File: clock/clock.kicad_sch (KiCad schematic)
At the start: 4 parts

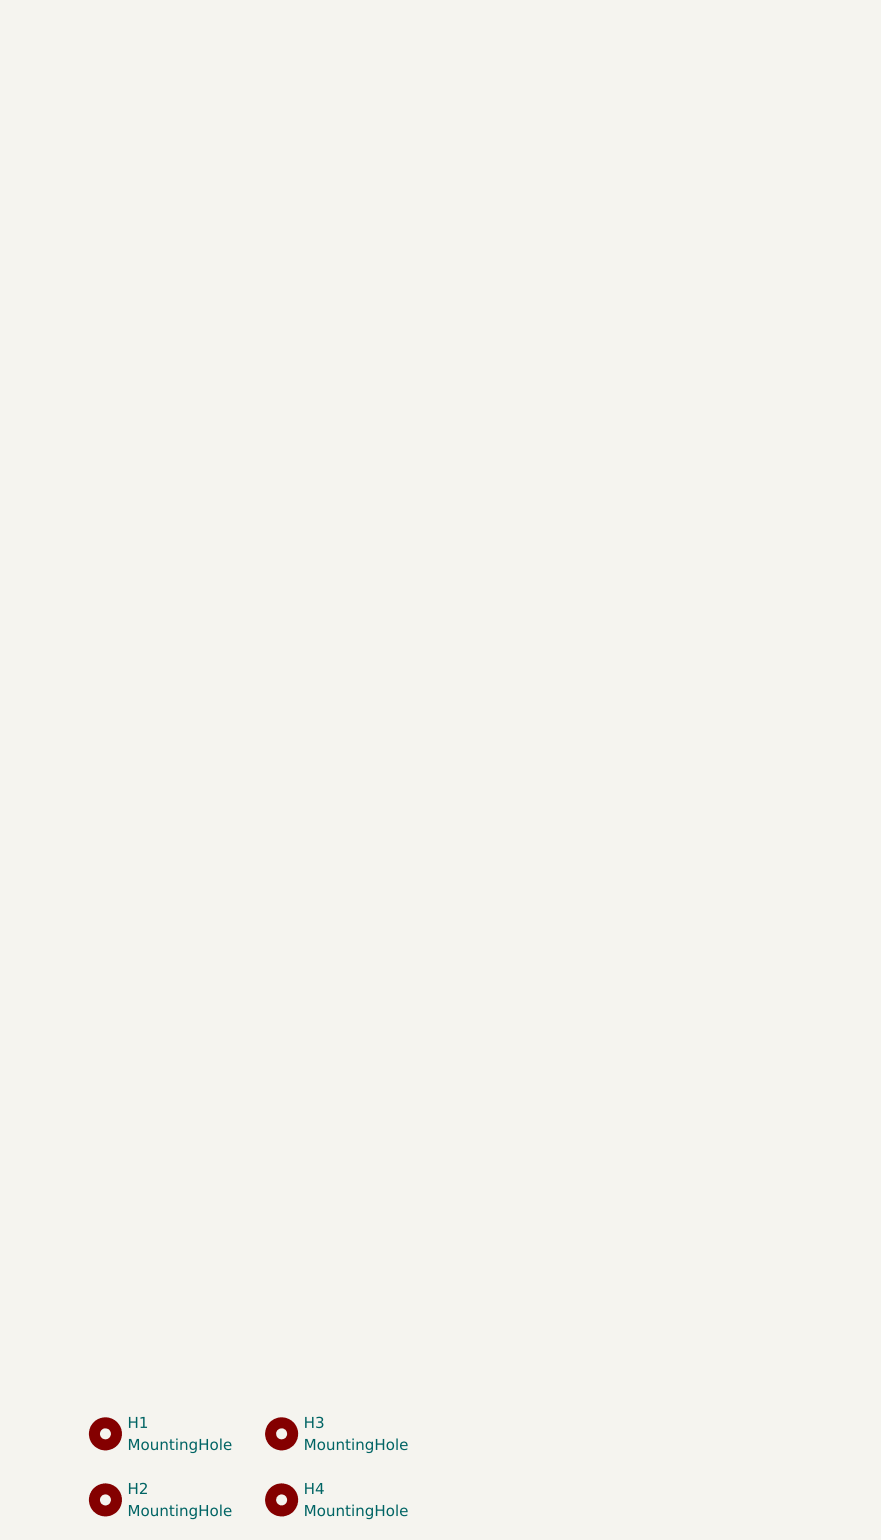
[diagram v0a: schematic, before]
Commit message: kinda week 2 deliverables
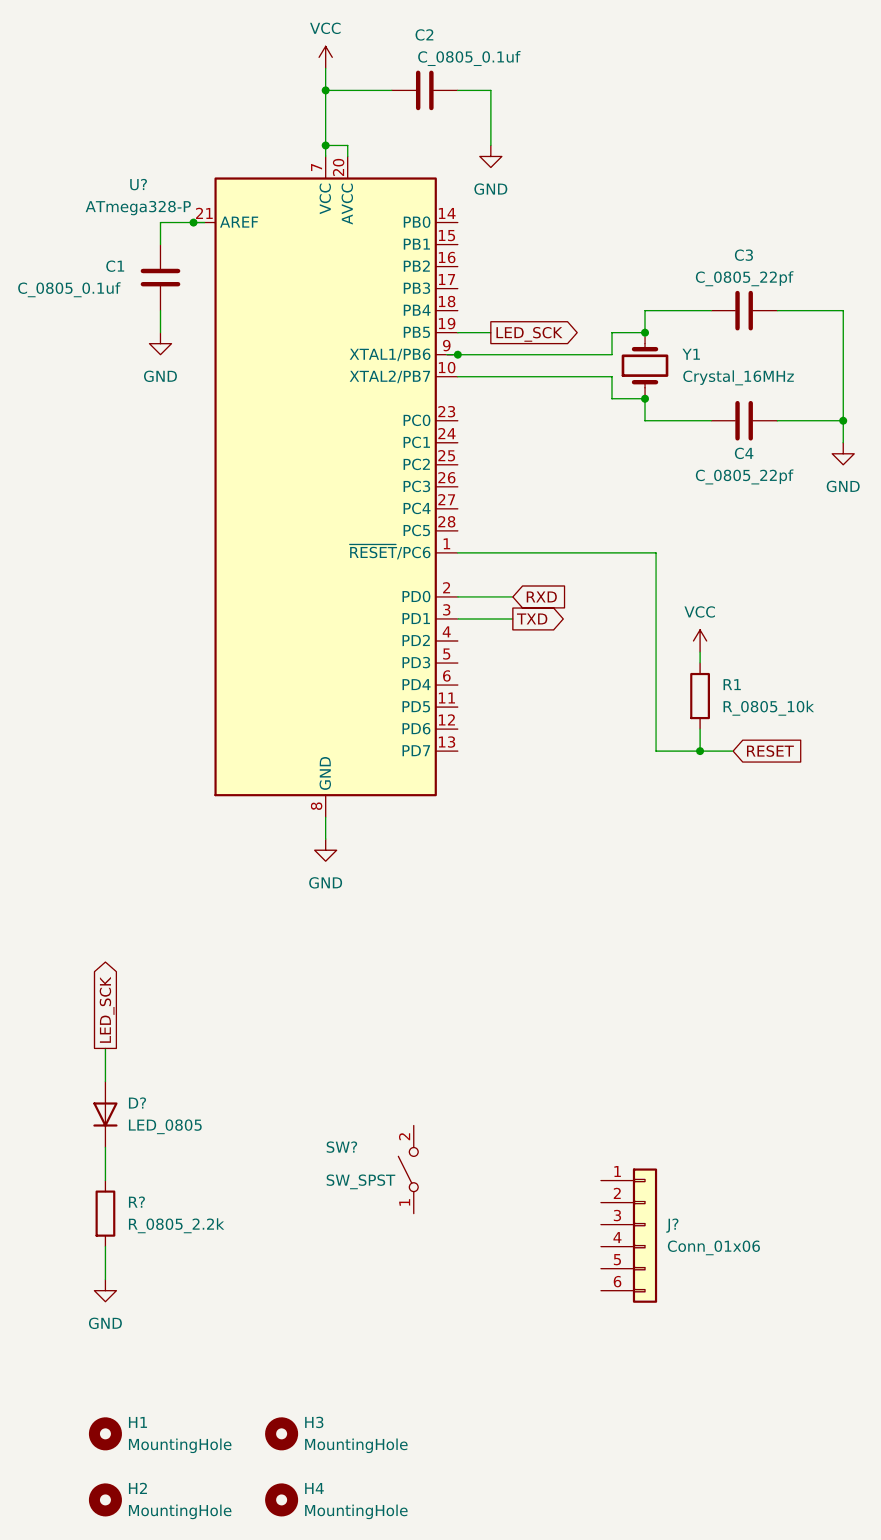
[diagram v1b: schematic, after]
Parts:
- added C1, C2: C_0805_0.1uf, symbol Device:C
- added C3, C4: C_0805_22pf, symbol Device:C
- added D?: LED_0805, symbol Device:D
- added J?: Conn_01x06, symbol Connector_Generic:Conn_01x06
- added R1: R_0805_10k, symbol Device:R
- added R?: R_0805_2.2k, symbol Device:R
- added SW?: SW_SPST, symbol Switch:SW_SPST
- added U?: ATmega328-P, Package_DIP:DIP-28_W7.62mm, symbol MCU_Microchip_ATmega:ATmega328-P
- added Y1: Crystal_16MHz, symbol Device:Crystal
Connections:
- new net: D?.1 (K), R?.1
- new net: C4.2, U?.10 (XTAL2/PB7), Y1.1
- new net: C1.1, U?.21 (AREF)
- new net: C3.1, U?.9 (XTAL1/PB6), Y1.2
- new net GND: C1.2, C2.2, C3.2, C4.1, R?.2, U?.22 (GND), U?.8 (GND)
- new net LED_SCK: D?.2 (A), U?.19 (PB5)
- new net RESET: R1.2, U?.1 (~{RESET}/PC6)
- new net RXD: U?.2 (PD0)
- new net TXD: U?.3 (PD1)
- new net VCC: C2.1, R1.1, U?.20 (AVCC), U?.7 (VCC)
